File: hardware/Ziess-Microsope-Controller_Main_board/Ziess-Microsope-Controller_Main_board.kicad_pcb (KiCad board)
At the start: 4 copper layers, 120 x 130 mm, 428 parts, among them IC1 TRS3122ERGER, J1 0430450606, J10 B3B-XH-AM, J11 B4B-XH-AM, J12 B2B-XH-AM, J13 B6B-XH-AM, J14 B6B-XH-AM, J15 B3B-XH-AM, J17 Conn_01x10, J18 B4B-XH-AM, J2 B4B-XH-AM, J20 031532951RFX, J21 Conn_01x10, J22 Conn_01x10, J3 B4B-XH-AM, J4 B2B-XH-AM, J5 B2B-XH-AM, J6 B2B-XH-AM, J7 B3B-XH-AM, J8 B3B-XH-AM, J9 B6B-XH-AM, Q1 BSS84, Q2 2N7002, Q3 2N7002, Q4 2N7002, SW1 RESET, SW2 SW_Push, SW3 CJS1201A, U1 TPS24751RUVR, U10 SN74LVC2G17DBV, U11 SN74LVC2G17DBV, U12 SN74LVC2G17DBV, U13 SN74LVC2G17DBV, U14 SN74LVC2G17DBV, U15 USBLC6-2SC6, U16 74LVC1G17, U18 STM32F765VGTx, U2 TPS54336ADDA, U20 TPS259472LRPWR, U21 TPS259472LRPWR, U3 AMS1117-3.3, U4 TPS2116DRL, U5 TMC2209-LA, U6 TMC2209-LA, U7 DRV8876PWPR, U8 DRV8876PWPR, U9 DRV8876PWPR, Y1 Crystal_Small

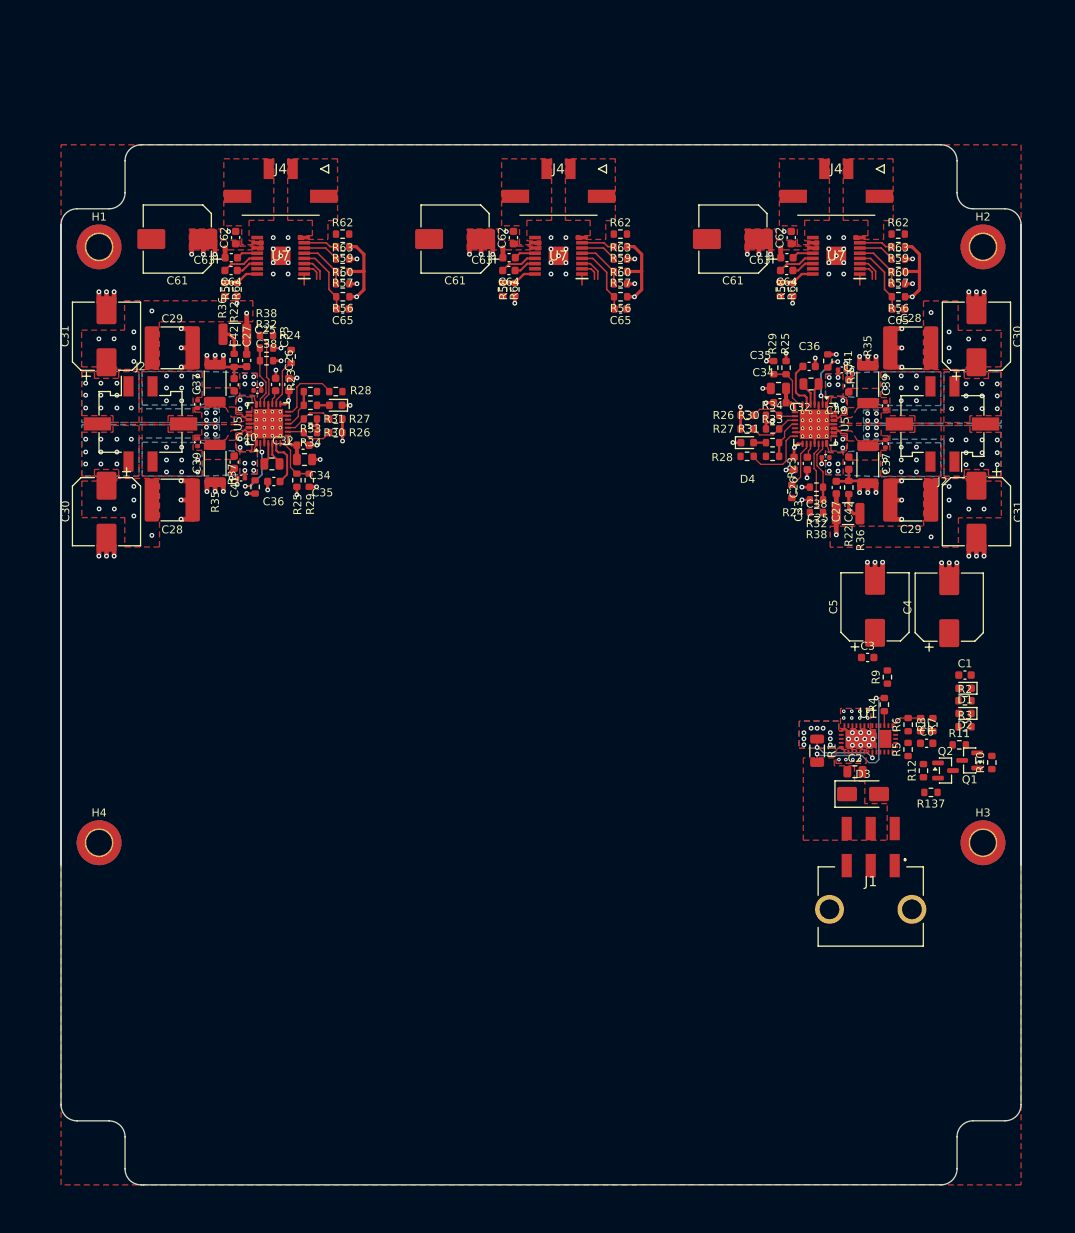
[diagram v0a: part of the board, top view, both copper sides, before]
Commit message: m
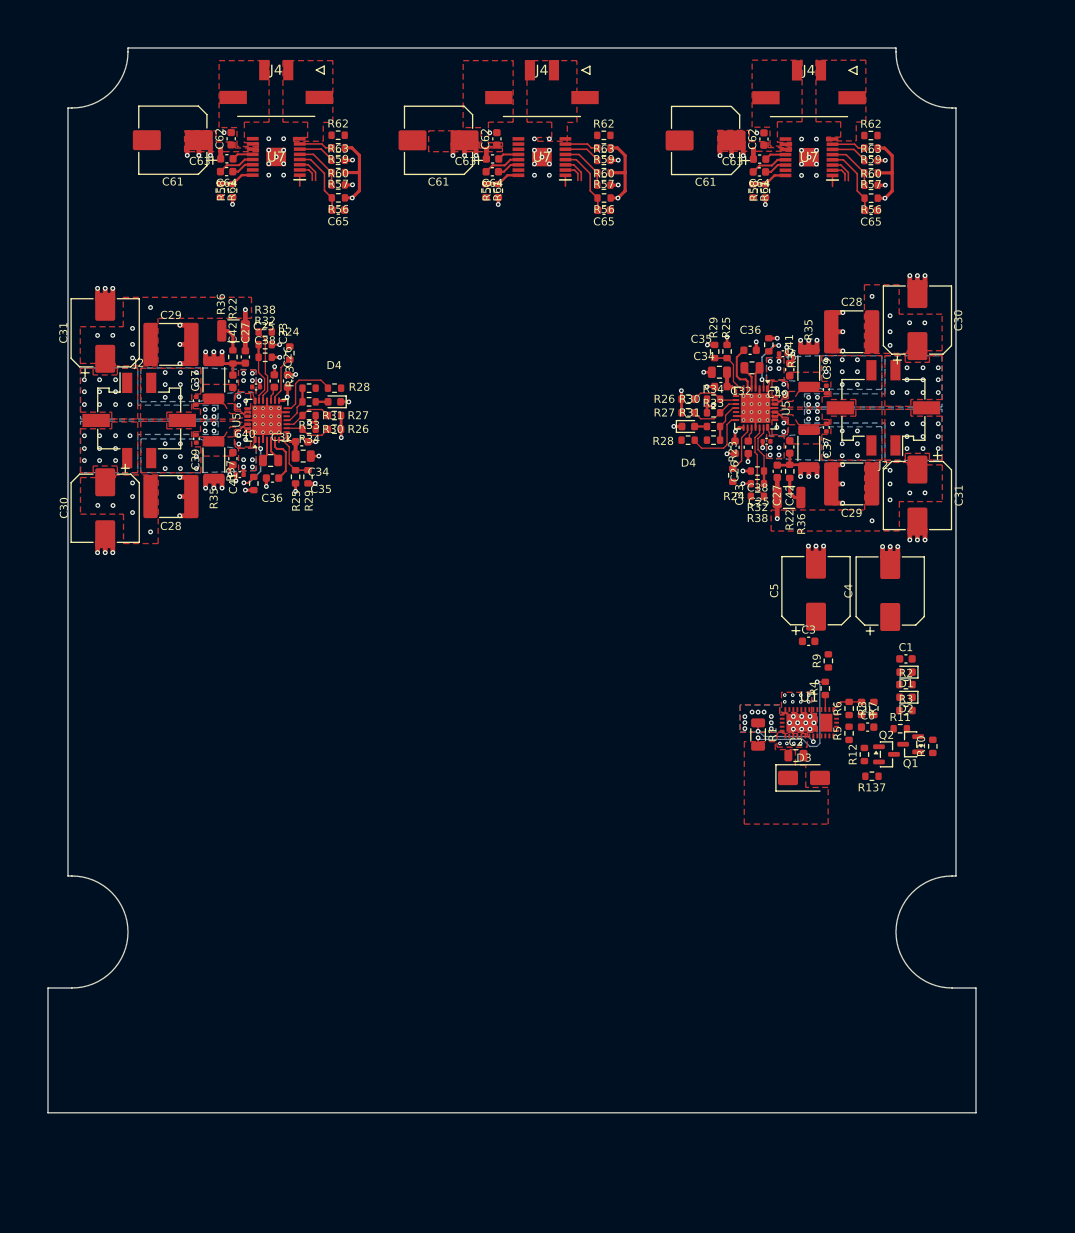
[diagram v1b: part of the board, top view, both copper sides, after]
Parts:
- removed the C61 at (168.0, 37.5)
- removed the C61 at (133.3, 37.5)
- removed the C62 at (140.6, 37.4)
- removed the C62 at (175.3, 37.4)
- removed the C63 at (140.1, 39.9)
- removed the C63 at (174.8, 39.9)
- removed the C64 at (140.0, 41.5)
- removed the C64 at (174.8, 41.5)
- removed the C65 at (188.7, 46.3)
- removed the C65 at (154.0, 46.3)
- removed H1, H2, H3, H4: MountingHole, MountingHole:MountingHole_3.2mm_M3_DIN965_Pad_TopBottom
- removed J1: 0430450606, Library:0430450606
- removed the J4 at (146.2, 28.8)
- removed the J4 at (181.0, 28.8)
- removed the R56 at (188.7, 44.7)
- removed the R56 at (154.0, 44.7)
- removed the R57 at (188.7, 41.6)
- removed the R57 at (154.0, 41.6)
- removed the R58 at (175.5, 43.8)
- removed the R58 at (140.8, 43.8)
- removed the R59 at (188.7, 38.5)
- removed the R59 at (154.0, 38.5)
- removed the R60 at (154.0, 43.1)
- removed the R60 at (188.7, 43.1)
- removed the R61 at (174.0, 43.8)
- removed the R61 at (139.2, 43.8)
- removed the R62 at (154.0, 36.9)
- removed the R62 at (188.7, 36.9)
- removed the R63 at (154.0, 40.0)
- removed the R63 at (188.7, 40.0)
- removed the U7 at (146.2, 39.6)
- removed the U7 at (181.0, 39.6)
- added C61: 220uF, Capacitor_SMD:CP_Elec_8x10, F.Cu at (131.2, 25.2)
- added C61: 220uF, Capacitor_SMD:CP_Elec_8x10, F.Cu at (164.6, 25.2)
- added C62: 100nF, Capacitor_SMD:C_0603_1608Metric, F.Cu at (138.5, 25.0)
- added C62: 100nF, Capacitor_SMD:C_0603_1608Metric, F.Cu at (171.9, 25.0)
- added C63: 100nF, Capacitor_SMD:C_0603_1608Metric, F.Cu at (138.0, 27.5)
- added C63: 100nF, Capacitor_SMD:C_0603_1608Metric, F.Cu at (171.4, 27.5)
- added C64: 22nF, Capacitor_SMD:C_0603_1608Metric, F.Cu at (171.4, 29.1)
- added C64: 22nF, Capacitor_SMD:C_0603_1608Metric, F.Cu at (138.0, 29.1)
- added C65: 100nF, Capacitor_SMD:C_0603_1608Metric, F.Cu at (185.3, 34.0)
- added C65: 100nF, Capacitor_SMD:C_0603_1608Metric, F.Cu at (151.9, 33.9)
- added J4: B2B-XH-AM, Library:43650-02YY_242526, F.Cu at (177.6, 16.4)
- added J4: B2B-XH-AM, Library:43650-02YY_242526, F.Cu at (144.2, 16.4)
- added R56: 10k, Resistor_SMD:R_0603_1608Metric, F.Cu at (151.9, 32.4)
- added R56: 10k, Resistor_SMD:R_0603_1608Metric, F.Cu at (185.3, 32.4)
- added R57: 1k, Resistor_SMD:R_0603_1608Metric, F.Cu at (185.3, 29.3)
- added R57: 1k, Resistor_SMD:R_0603_1608Metric, F.Cu at (151.9, 29.2)
- added R58: 0, Resistor_SMD:R_0603_1608Metric, F.Cu at (138.7, 31.5)
- added R58: 0, Resistor_SMD:R_0603_1608Metric, F.Cu at (172.1, 31.5)
- added R59: 0, Resistor_SMD:R_0603_1608Metric, F.Cu at (151.9, 26.1)
- added R59: 0, Resistor_SMD:R_0603_1608Metric, F.Cu at (185.3, 26.2)
- added R60: 11k, Resistor_SMD:R_0603_1608Metric, F.Cu at (185.3, 30.8)
- added R60: 11k, Resistor_SMD:R_0603_1608Metric, F.Cu at (151.9, 30.8)
- added R61: 0, Resistor_SMD:R_0603_1608Metric, F.Cu at (137.2, 31.5)
- added R61: 0, Resistor_SMD:R_0603_1608Metric, F.Cu at (170.6, 31.5)
- added R62: 0, Resistor_SMD:R_0603_1608Metric, F.Cu at (185.3, 24.6)
- added R62: 0, Resistor_SMD:R_0603_1608Metric, F.Cu at (151.9, 24.6)
- added R63: 6.8k, Resistor_SMD:R_0603_1608Metric, F.Cu at (151.9, 27.7)
- added R63: 6.8k, Resistor_SMD:R_0603_1608Metric, F.Cu at (185.3, 27.7)
- added U7: DRV8876PWPR, Library:SOP65P640X120-17N, F.Cu at (144.2, 27.3)
- added U7: DRV8876PWPR, Library:SOP65P640X120-17N, F.Cu at (177.6, 27.3)
- moved C61 12.4 mm to (98.0, 25.2)
- moved C62 12.4 mm to (105.3, 25.0)
- moved C65 12.4 mm to (118.7, 33.9)
- moved R56 12.4 mm to (118.7, 32.4)
- moved R59 12.4 mm to (118.7, 26.1)
- moved R60 12.4 mm to (118.7, 30.8)
- moved R62 12.4 mm to (118.7, 24.6)
- moved C63 12.4 mm to (104.8, 27.5)
- moved C64 12.4 mm to (104.8, 29.1)
- moved J4 12.4 mm to (111.0, 16.4)
- moved R57 12.4 mm to (118.7, 29.2)
- moved R58 12.4 mm to (105.5, 31.5)
- moved R61 12.4 mm to (104.0, 31.5)
- moved R63 12.4 mm to (118.7, 27.7)
- moved U7 12.4 mm to (111.0, 27.3)
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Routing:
- removed copper zone on In2.Cu, net +12V
- removed copper zone on In1.Cu, net GND
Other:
- board size 120 x 130 mm -> 116 x 133.1 mm
